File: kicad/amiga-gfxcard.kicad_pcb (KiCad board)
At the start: 2 copper layers, 29 parts, among them P1 ADDR1, P2 ADDR2, P3 ADDR3, P4 DATA1, P5 DATA2, P6 CTRL_IN, P7 CTRL_OUT, U1 74LVC8T245, U2 74LVC8T245, U3 74LVC8T245, U4 74LVC8T245, U5 74LVC8T245, U6 74LVC8T245

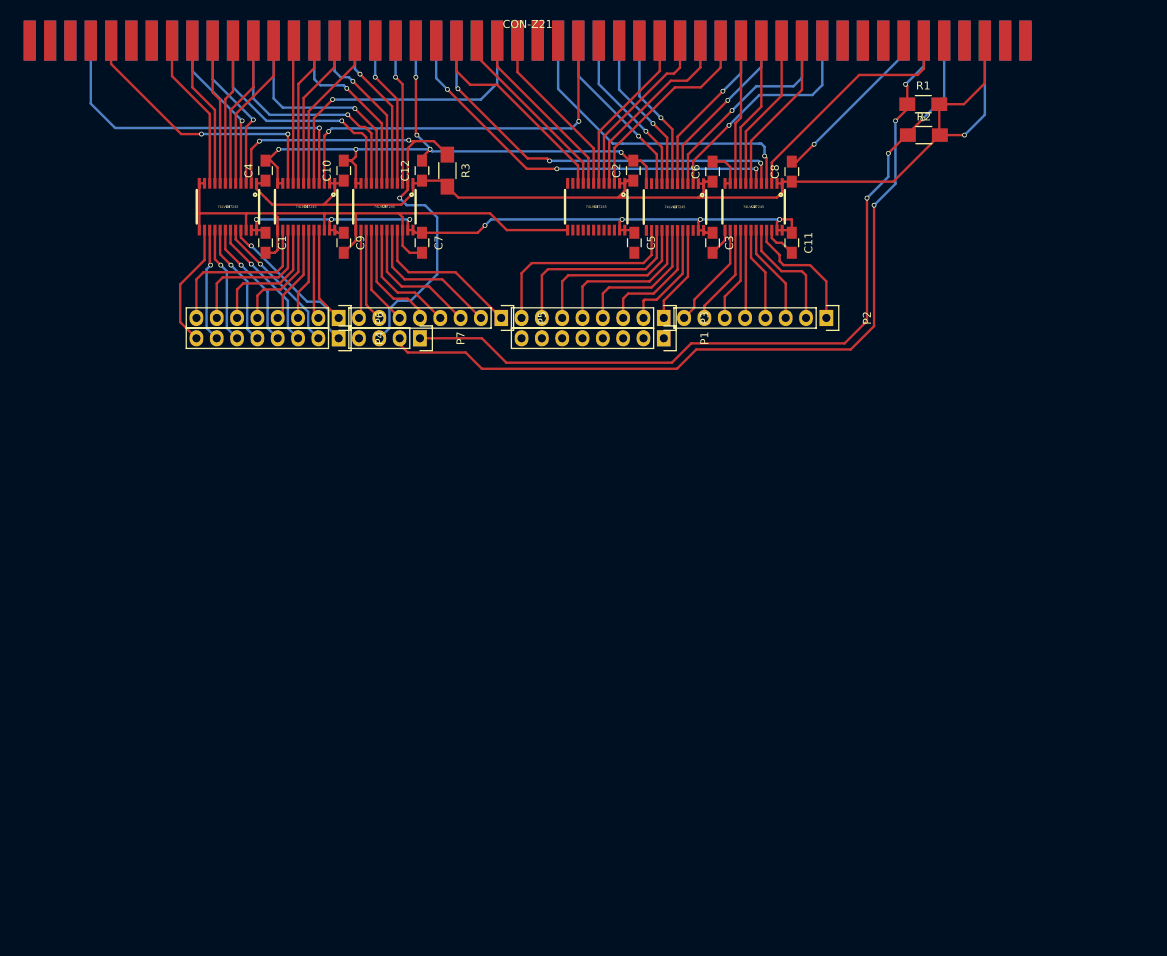
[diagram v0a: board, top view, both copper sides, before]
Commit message: redo of mk2 board finished
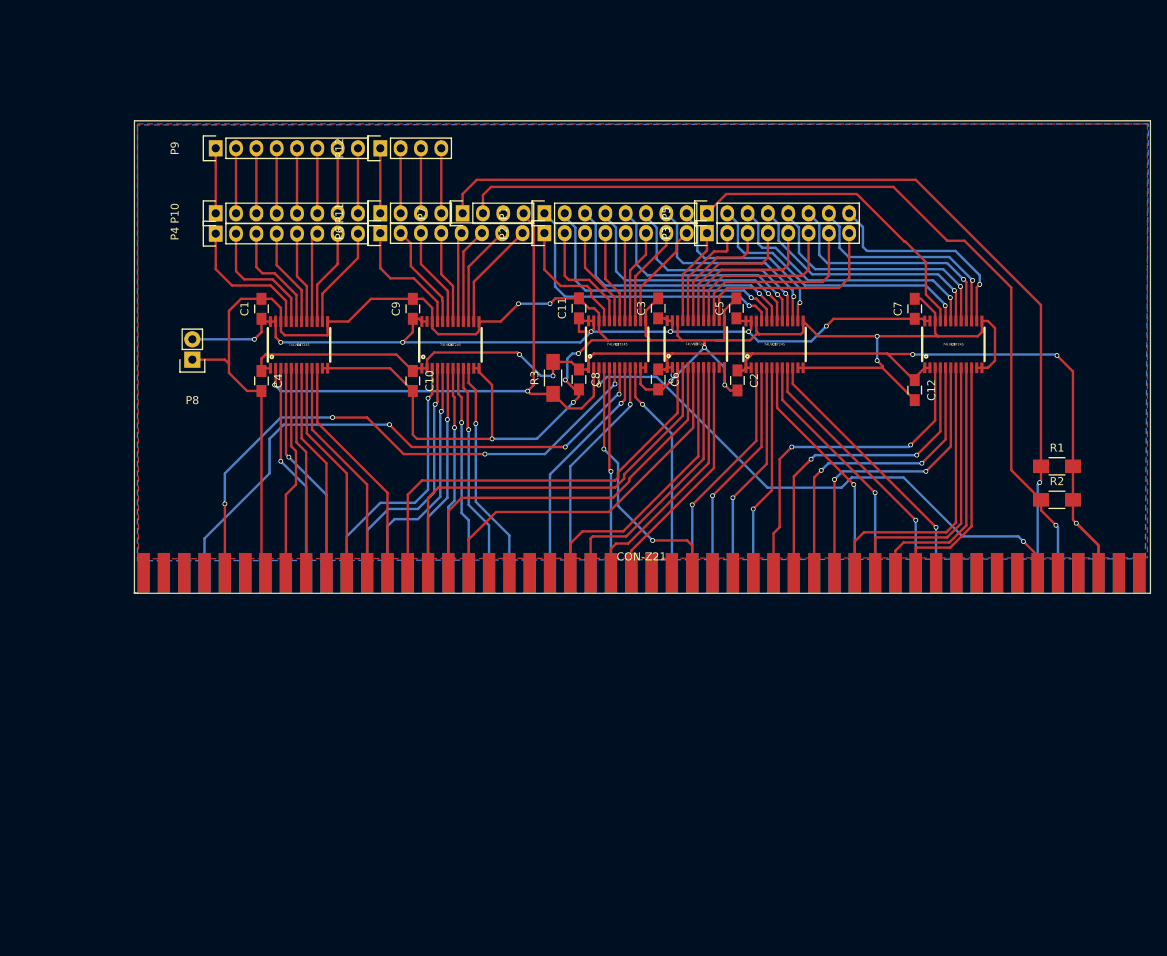
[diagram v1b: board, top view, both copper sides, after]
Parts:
- added P10: AUX1B, Pin_Headers:Pin_Header_Straight_1x08, F.Cu at (111.5, 48.8)
- added P11: AUX2A, Pin_Headers:Pin_Header_Straight_1x04, F.Cu at (132.1, 48.8)
- added P12: AUX2B, Pin_Headers:Pin_Header_Straight_1x04, F.Cu at (132.1, 40.6)
- added P8: CONN_01X02, Pin_Headers:Pin_Header_Straight_1x02, F.Cu at (108.6, 67.1)
- added P9: AUX1A, Pin_Headers:Pin_Header_Straight_1x08, F.Cu at (111.5, 40.6)
- P3: value ADDR3 -> ADDR4
- P4: value DATA1 -> DATA2
- P5: value DATA2 -> ADDR3
- P6: value CTRL_IN -> DATA1
- moved U5 73.2 mm to (203.7, 65.2), turned to 0 degrees
- moved CON-Z21 68.1 mm to (164.7, 91.2)
- moved C12 67.4 mm to (198.9, 70.9), turned to 270 degrees
- moved C7 62.1 mm to (198.9, 60.7), turned to 90 degrees
- moved R2 48.5 mm to (216.7, 84.6)
- moved R1 48.2 mm to (216.7, 80.4)
- moved C8 37.2 mm to (156.9, 69.5), turned to 270 degrees
- moved P2 36.8 mm to (152.6, 51.2), turned to 90 degrees
- moved C2 29.3 mm to (176.7, 69.7), turned to 270 degrees
- moved R3 29.1 mm to (153.7, 69.3), turned to 90 degrees
- moved P5 28.9 mm to (172.9, 48.8), turned to 90 degrees
- moved U1 28.2 mm to (181.4, 65.2), turned to 0 degrees
- moved C11 27.8 mm to (156.9, 60.6), turned to 90 degrees
- moved C10 27.7 mm to (136.1, 69.7), turned to 270 degrees
- moved C6 26.8 mm to (166.8, 69.5), turned to 270 degrees
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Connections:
- P7 pad 1: Net-(CON-Z21-Pad9) -> Net-(CON-Z21-Pad11)
- P7 pad 2: Net-(CON-Z21-Pad11) -> Net-(CON-Z21-Pad9)
- R3 pad 1: Net-(P7-Pad3) -> Net-(P7-Pad4)
- U1 pad 10: Net-(CON-Z21-Pad58) -> Net-(CON-Z21-Pad21)
- U1 pad 3: Net-(CON-Z21-Pad32) -> Net-(CON-Z21-Pad45)
- U1 pad 4: Net-(CON-Z21-Pad34) -> Net-(CON-Z21-Pad43)
- U1 pad 5: Net-(CON-Z21-Pad36) -> Net-(CON-Z21-Pad41)
- U1 pad 6: Net-(CON-Z21-Pad38) -> Net-(CON-Z21-Pad39)
- U1 pad 7: Net-(CON-Z21-Pad52) -> Net-(CON-Z21-Pad29)
- U1 pad 8: Net-(CON-Z21-Pad54) -> Net-(CON-Z21-Pad27)
- U1 pad 9: Net-(CON-Z21-Pad56) -> Net-(CON-Z21-Pad23)
- U2 pad 10: Net-(CON-Z21-Pad30) -> Net-(CON-Z21-Pad47)
- U2 pad 2: +5V -> Net-(P7-Pad4)
- U2 pad 4: Net-(CON-Z21-Pad47) -> Net-(CON-Z21-Pad46)
- U2 pad 5: Net-(CON-Z21-Pad57) -> Net-(CON-Z21-Pad53)
- U2 pad 6: Net-(CON-Z21-Pad59) -> Net-(CON-Z21-Pad92)
- U2 pad 7: Net-(CON-Z21-Pad24) -> Net-(CON-Z21-Pad93)
- U2 pad 8: Net-(CON-Z21-Pad26) -> Net-(CON-Z21-Pad59)
- U2 pad 9: Net-(CON-Z21-Pad28) -> Net-(CON-Z21-Pad57)
- U3 pad 10: Net-(CON-Z21-Pad45) -> Net-(CON-Z21-Pad52)
- U3 pad 3: Net-(CON-Z21-Pad21) -> Net-(CON-Z21-Pad74)
- U3 pad 4: Net-(CON-Z21-Pad23) -> Net-(CON-Z21-Pad72)
- U3 pad 5: Net-(CON-Z21-Pad27) -> Net-(CON-Z21-Pad70)
- U3 pad 6: Net-(CON-Z21-Pad29) -> Net-(CON-Z21-Pad68)
- U3 pad 7: Net-(CON-Z21-Pad39) -> Net-(CON-Z21-Pad58)
- U3 pad 8: Net-(CON-Z21-Pad41) -> Net-(CON-Z21-Pad56)
- U3 pad 9: Net-(CON-Z21-Pad43) -> Net-(CON-Z21-Pad54)
- U4 pad 10: Net-(CON-Z21-Pad86) -> Net-(CON-Z21-Pad76)
- U4 pad 2: Net-(P7-Pad3) -> Net-(P7-Pad4)
- U4 pad 3: Net-(CON-Z21-Pad81) -> Net-(CON-Z21-Pad83)
- U4 pad 4: Net-(CON-Z21-Pad83) -> Net-(CON-Z21-Pad81)
- U4 pad 5: Net-(CON-Z21-Pad76) -> Net-(CON-Z21-Pad86)
- U4 pad 6: Net-(CON-Z21-Pad78) -> Net-(CON-Z21-Pad84)
- U4 pad 7: Net-(CON-Z21-Pad80) -> Net-(CON-Z21-Pad82)
- U4 pad 8: Net-(CON-Z21-Pad82) -> Net-(CON-Z21-Pad80)
- U4 pad 9: Net-(CON-Z21-Pad84) -> Net-(CON-Z21-Pad78)
- U5 pad 10: Net-(CON-Z21-Pad79) -> Net-(CON-Z21-Pad24)
- U5 pad 2: Net-(P7-Pad3) -> +5V
- U5 pad 3: Net-(CON-Z21-Pad63) -> Net-(CON-Z21-Pad38)
- U5 pad 4: Net-(CON-Z21-Pad65) -> Net-(CON-Z21-Pad36)
- U5 pad 5: Net-(CON-Z21-Pad67) -> Net-(CON-Z21-Pad34)
- U5 pad 6: Net-(CON-Z21-Pad69) -> Net-(CON-Z21-Pad32)
- U5 pad 7: Net-(CON-Z21-Pad71) -> Net-(CON-Z21-Pad30)
- U5 pad 8: Net-(CON-Z21-Pad75) -> Net-(CON-Z21-Pad28)
- U5 pad 9: Net-(CON-Z21-Pad77) -> Net-(CON-Z21-Pad26)
- U6 pad 10: Net-(CON-Z21-Pad92) -> Net-(CON-Z21-Pad63)
- U6 pad 3: Net-(CON-Z21-Pad46) -> Net-(CON-Z21-Pad79)
- U6 pad 4: Net-(CON-Z21-Pad93) -> Net-(CON-Z21-Pad77)
- U6 pad 5: Net-(CON-Z21-Pad53) -> Net-(CON-Z21-Pad75)
- U6 pad 6: Net-(CON-Z21-Pad68) -> Net-(CON-Z21-Pad71)
- U6 pad 7: Net-(CON-Z21-Pad70) -> Net-(CON-Z21-Pad69)
- U6 pad 8: Net-(CON-Z21-Pad72) -> Net-(CON-Z21-Pad67)
- U6 pad 9: Net-(CON-Z21-Pad74) -> Net-(CON-Z21-Pad65)
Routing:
- net GND: track 190.3 -> 296.8 mm, vias 7 -> 11
- net Net-(P7-Pad4): track 0.00 -> 70.5 mm, vias 0 -> 2
- net Net-(P7-Pad3): track 62.7 -> 0.00 mm, vias 3 -> 0
- net Net-(CON-Z21-Pad12): track 30.0 -> 69.9 mm, vias 0 -> 2
- net Net-(P1-Pad1): track 0.00 -> 37.9 mm, vias 0 -> 1
- net Net-(CON-Z21-Pad92): track 34.8 -> 71.7 mm, vias 2 -> 4
- net Net-(CON-Z21-Pad74): track 17.9 -> 53.8 mm
- net Net-(P1-Pad2): track 0.00 -> 35.8 mm, vias 0 -> 1
- net Net-(P1-Pad3): track 0.00 -> 33.8 mm, vias 0 -> 1
- net Net-(CON-Z21-Pad72): track 18.7 -> 51.8 mm
- net Net-(P1-Pad4): track 0.00 -> 31.9 mm, vias 0 -> 1
- net +3V3: track 88.7 -> 118.4 mm
- net Net-(CON-Z21-Pad70): track 19.4 -> 49.2 mm
- net Net-(P1-Pad5): track 0.00 -> 29.7 mm, vias 0 -> 1
- net Net-(P1-Pad6): track 0.00 -> 27.7 mm, vias 0 -> 1
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- added copper zone on B.Cu, net GND
- added copper zone on F.Cu, net GND
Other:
- board outline added: 127 x 59.1 mm

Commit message: board v1.2 finished
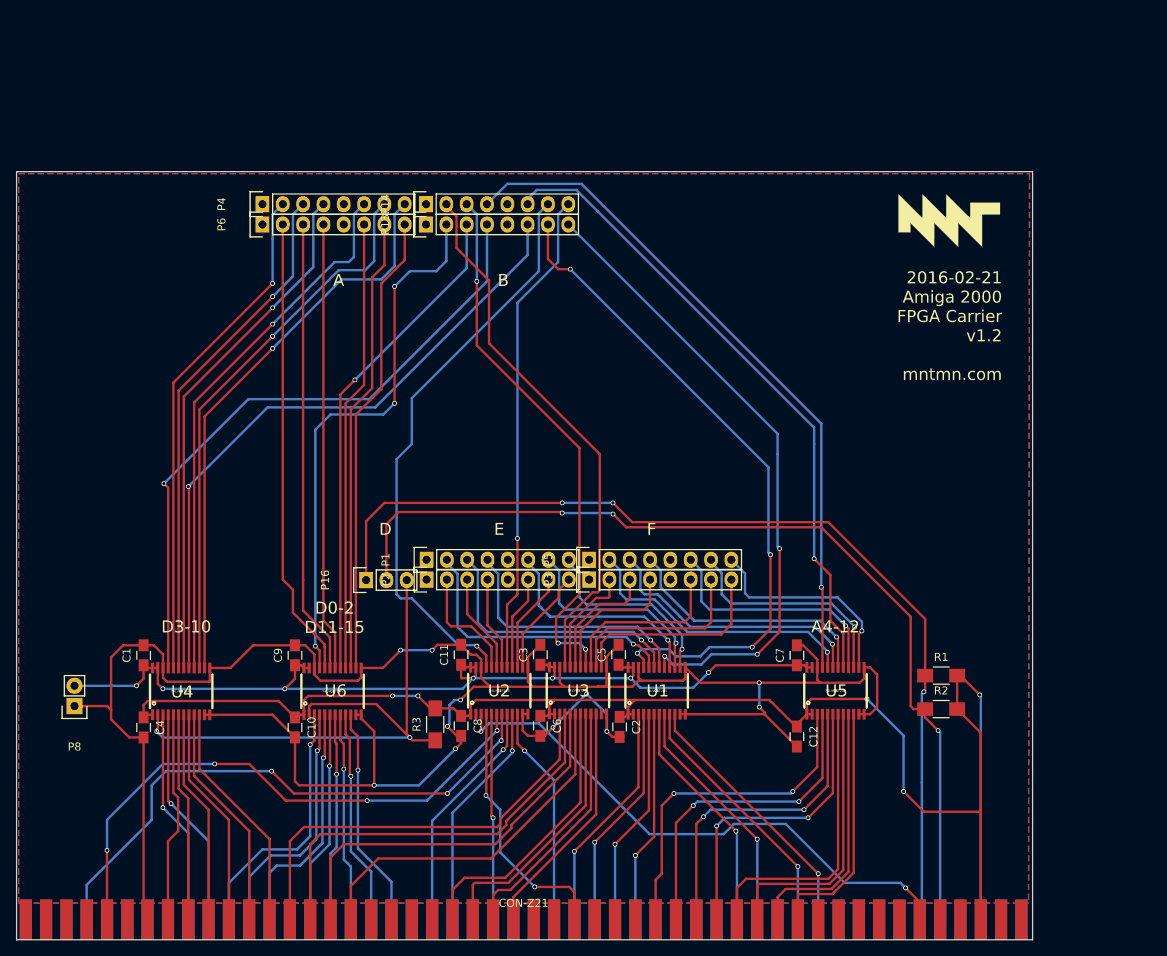
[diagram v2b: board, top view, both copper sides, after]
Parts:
- removed P10: AUX1B, Pin_Headers:Pin_Header_Straight_1x08
- removed P11: AUX2A, Pin_Headers:Pin_Header_Straight_1x04
- removed P12: AUX2B, Pin_Headers:Pin_Header_Straight_1x04
- removed P7: CTRL_OUT, Pin_Headers:Pin_Header_Straight_1x04
- removed P9: AUX1A, Pin_Headers:Pin_Header_Straight_1x08
- added G***: LOGO, mnt:mnt, F.Cu at (203.2, 49.7)
- added P13: X1, Pin_Headers:Pin_Header_Straight_1x08, F.Cu at (137.8, 50.2)
- added P14: X2, Pin_Headers:Pin_Header_Straight_1x08, F.Cu at (137.8, 47.6)
- added P16: D1, Pin_Headers:Pin_Header_Straight_1x03, F.Cu at (130.3, 94.6)
- moved C1 45.7 mm to (102.5, 104.0)
- moved C10 45.7 mm to (121.4, 113.0)
- moved C11 45.7 mm to (142.2, 103.9)
- moved C12 45.7 mm to (184.2, 114.2)
- moved C2 45.7 mm to (162.0, 113.0)
- moved C3 45.7 mm to (152.1, 103.9)
- moved C4 45.7 mm to (102.5, 113.0)
- moved C5 45.7 mm to (161.9, 103.9)
- moved C6 45.7 mm to (152.1, 112.8)
- moved C7 45.7 mm to (184.2, 104.0)
- moved C8 45.7 mm to (142.2, 112.8)
- moved C9 45.7 mm to (121.4, 104.0)
- moved P1 45.7 mm to (137.9, 92.1)
- moved P2 45.7 mm to (137.9, 94.6)
- moved P3 45.7 mm to (158.2, 94.6)
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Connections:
- CON-Z21 pad 10: Net-(CON-Z21-Pad10) -> (no net)
- CON-Z21 pad 14: Net-(CON-Z21-Pad14) -> (no net)
- CON-Z21 pad 15: Net-(CON-Z21-Pad15) -> (no net)
- CON-Z21 pad 16: Net-(CON-Z21-Pad16) -> (no net)
- CON-Z21 pad 17: Net-(CON-Z21-Pad17) -> (no net)
- CON-Z21 pad 18: Net-(CON-Z21-Pad18) -> (no net)
- CON-Z21 pad 19: Net-(CON-Z21-Pad19) -> (no net)
- CON-Z21 pad 20: Net-(CON-Z21-Pad20) -> (no net)
- CON-Z21 pad 22: Net-(CON-Z21-Pad22) -> (no net)
- CON-Z21 pad 31: Net-(CON-Z21-Pad31) -> (no net)
- CON-Z21 pad 33: Net-(CON-Z21-Pad33) -> (no net)
- CON-Z21 pad 35: Net-(CON-Z21-Pad35) -> (no net)
- CON-Z21 pad 40: Net-(CON-Z21-Pad40) -> (no net)
- CON-Z21 pad 42: Net-(CON-Z21-Pad42) -> (no net)
- CON-Z21 pad 44: Net-(CON-Z21-Pad44) -> (no net)
- CON-Z21 pad 48: Net-(CON-Z21-Pad48) -> (no net)
- CON-Z21 pad 50: Net-(CON-Z21-Pad50) -> (no net)
- CON-Z21 pad 51: Net-(CON-Z21-Pad51) -> (no net)
- CON-Z21 pad 55: Net-(CON-Z21-Pad55) -> (no net)
- CON-Z21 pad 60: Net-(CON-Z21-Pad60) -> (no net)
- CON-Z21 pad 62: Net-(CON-Z21-Pad62) -> (no net)
- CON-Z21 pad 64: Net-(CON-Z21-Pad64) -> (no net)
- CON-Z21 pad 66: Net-(CON-Z21-Pad66) -> (no net)
- CON-Z21 pad 7: Net-(CON-Z21-Pad7) -> (no net)
- CON-Z21 pad 8: Net-(CON-Z21-Pad8) -> (no net)
- CON-Z21 pad 91: Net-(CON-Z21-Pad91) -> (no net)
- CON-Z21 pad 94: Net-(CON-Z21-Pad94) -> (no net)
- CON-Z21 pad 95: Net-(CON-Z21-Pad95) -> (no net)
- CON-Z21 pad 96: Net-(CON-Z21-Pad96) -> (no net)
- CON-Z21 pad 97: Net-(CON-Z21-Pad97) -> (no net)
- CON-Z21 pad 98: Net-(CON-Z21-Pad98) -> (no net)
- P1 pad 1: Net-(P1-Pad1) -> (no net)
- P1 pad 5: Net-(P1-Pad5) -> (no net)
- P2 pad 1: Net-(P2-Pad1) -> (no net)
- P2 pad 5: Net-(P2-Pad5) -> (no net)
- P3 pad 1: Net-(P3-Pad1) -> (no net)
- P3 pad 5: Net-(P3-Pad5) -> (no net)
- P4 pad 1: Net-(P4-Pad1) -> (no net)
- P4 pad 5: Net-(P4-Pad5) -> (no net)
- P5 pad 1: Net-(P5-Pad1) -> (no net)
- P5 pad 5: Net-(P5-Pad5) -> (no net)
- P6 pad 1: Net-(P6-Pad1) -> (no net)
- P6 pad 5: Net-(P6-Pad5) -> (no net)
- R3 pad 1: Net-(P7-Pad4) -> Net-(P16-Pad3)
- U1 pad 17: Net-(P1-Pad5) -> Net-(P13-Pad8)
- U1 pad 21: Net-(P1-Pad1) -> Net-(P13-Pad7)
- U2 pad 17: Net-(P2-Pad5) -> Net-(P14-Pad8)
- U2 pad 2: Net-(P7-Pad4) -> +5V
- U2 pad 21: Net-(P2-Pad1) -> Net-(P14-Pad7)
- U3 pad 17: Net-(P3-Pad5) -> Net-(P14-Pad3)
- U3 pad 21: Net-(P3-Pad1) -> Net-(P14-Pad2)
- U4 pad 17: Net-(P4-Pad5) -> Net-(P13-Pad6)
- U4 pad 2: Net-(P7-Pad4) -> Net-(P16-Pad3)
- U4 pad 21: Net-(P4-Pad1) -> Net-(P13-Pad4)
- U5 pad 17: Net-(P5-Pad5) -> Net-(P14-Pad6)
- U5 pad 21: Net-(P5-Pad1) -> Net-(P14-Pad4)
- U6 pad 17: Net-(P6-Pad5) -> Net-(P13-Pad3)
- U6 pad 2: +5V -> Net-(P16-Pad3)
- U6 pad 21: Net-(P6-Pad1) -> Net-(P13-Pad2)
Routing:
- net Net-(P14-Pad4): track 0.00 -> 85.8 mm, vias 0 -> 1
- net Net-(P13-Pad7): track 0.00 -> 83.7 mm, vias 0 -> 4
- net Net-(P13-Pad4): track 0.00 -> 81.2 mm, vias 0 -> 1
- net Net-(P13-Pad6): track 0.00 -> 80.9 mm, vias 0 -> 1
- net Net-(P14-Pad6): track 0.00 -> 80.7 mm, vias 0 -> 1
- net Net-(P13-Pad8): track 0.00 -> 79.7 mm, vias 0 -> 3
- net Net-(P16-Pad3): track 0.00 -> 72.8 mm, vias 0 -> 2
- net Net-(P14-Pad7): track 0.00 -> 72.5 mm, vias 0 -> 1
- net Net-(P7-Pad4): track 70.5 -> 0.00 mm, vias 2 -> 0
- net Net-(P13-Pad2): track 0.00 -> 68.2 mm, vias 0 -> 3
- net Net-(P14-Pad3): track 0.00 -> 68.0 mm, vias 0 -> 3
- net Net-(P14-Pad2): track 0.00 -> 68.0 mm
- net Net-(P13-Pad3): track 0.00 -> 62.0 mm, vias 0 -> 1
- net Net-(P14-Pad8): track 0.00 -> 61.1 mm, vias 0 -> 1
- net Net-(P4-Pad8): track 12.8 -> 71.2 mm, vias 0 -> 1
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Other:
- board size 127 x 59.1 mm -> 127 x 96 mm
- board text added: "2016-02-21 Amiga 2000 FPGA Carrier v1.2 mntmn.com"
- board text added: "A"
- board text added: "A4-12"
- board text added: "B"
- board text added: "D"
- board text added: "D0-2 D11-15"
- board text added: "D3-10"
- board text added: "E"
- board text added: "F"
- board text added: "U1"
- board text added: "U2"
- board text added: "U3"
- board text added: "U4"
- board text added: "U5"
- board text added: "U6"
